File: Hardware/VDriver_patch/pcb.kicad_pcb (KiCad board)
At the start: 4 copper layers, 39.6 x 41.9 mm, 88 parts, among them J501 KAI11002_top, J502 Conn_01x02, J503 Conn_01x02, J504 Conn_01x02, J505 Conn_01x02, J506 Conn_02x05_Odd_Even, U514 1EDN7550B, U515 1EDN7550B, U516 1EDN7550B, U517 1EDN7550B, U518 IRF9389/7309, U519 IRF9389/7309, U520 IRF9389/7309

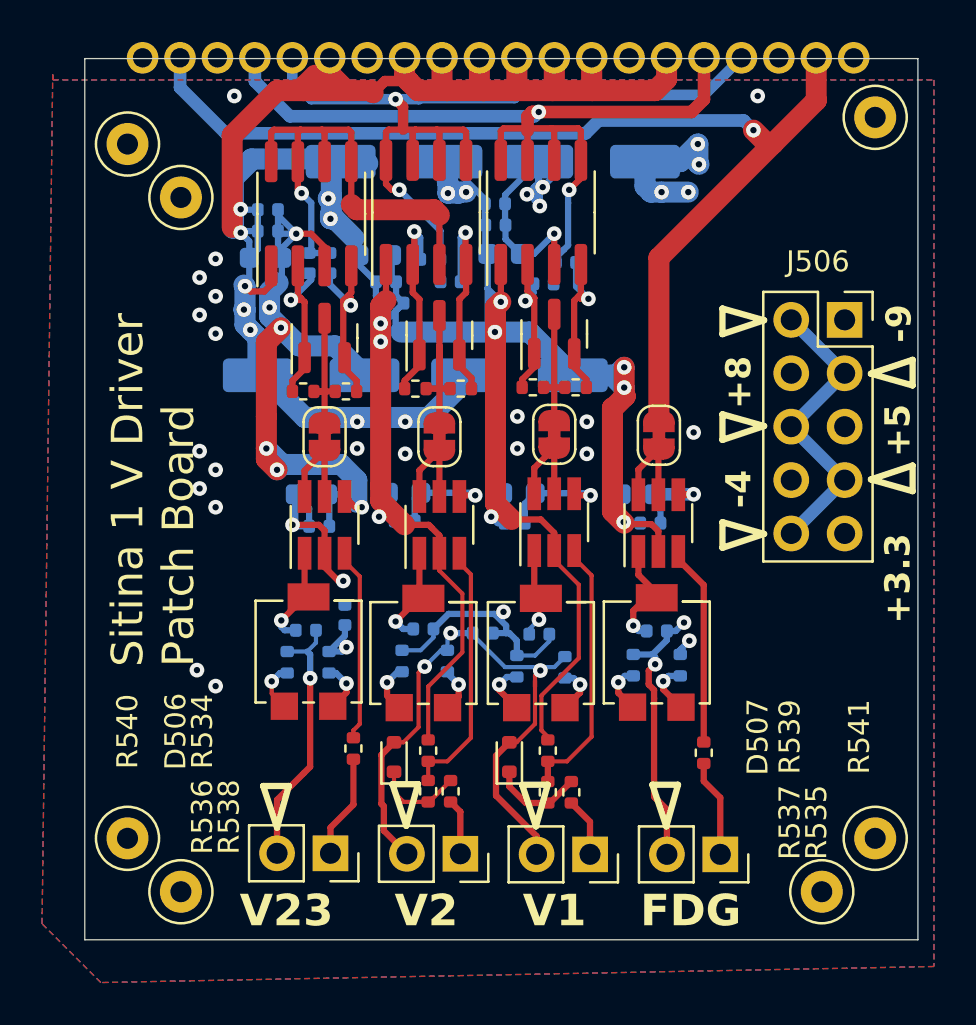
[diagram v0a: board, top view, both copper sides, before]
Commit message: Power Board WIP
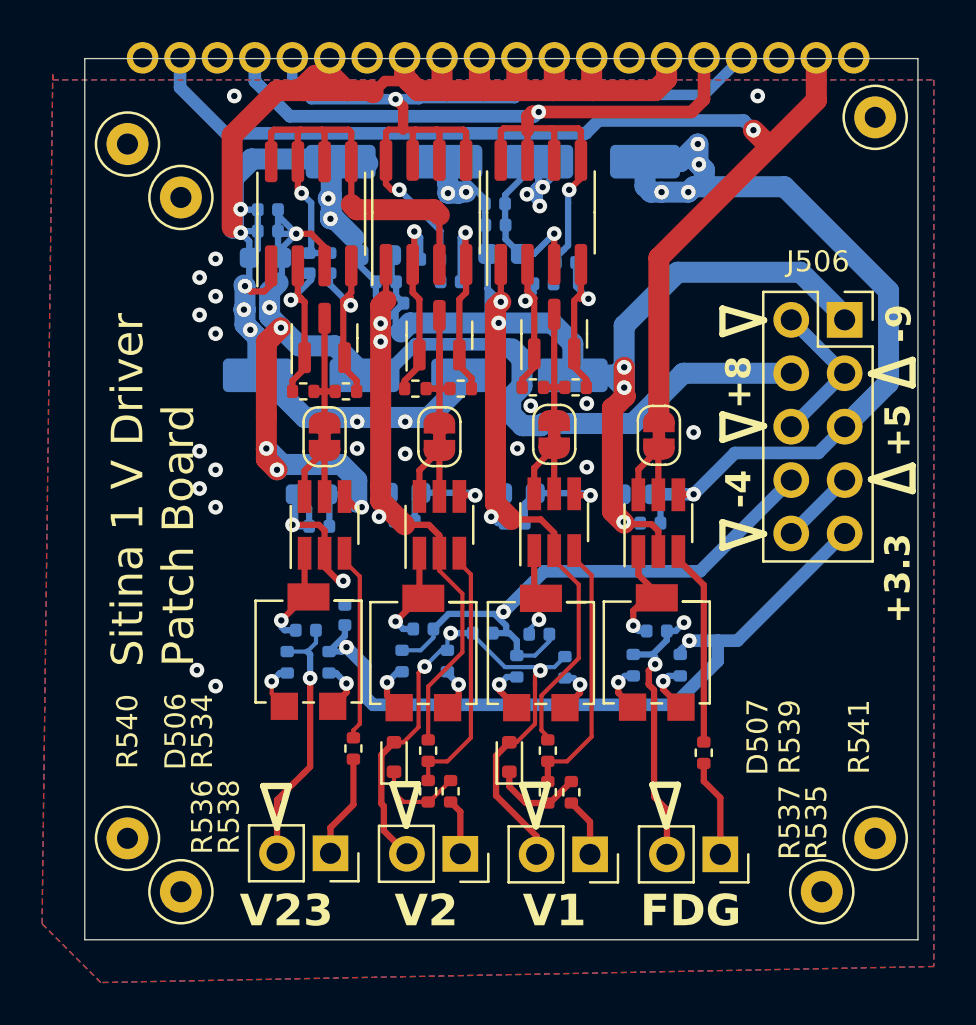
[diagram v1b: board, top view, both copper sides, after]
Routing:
- net +8V: track 35.5 -> 61.3 mm
- net +5V: track 20.7 -> 40.8 mm
- net -9V: track 104.3 -> 120.7 mm
- net +3V3: track 30.0 -> 34.3 mm
- net GND: track 188.1 -> 184.5 mm
- removed copper zone on In1.Cu, net +5V
- removed copper zone on In2.Cu, net +5V
- removed copper zone on In1.Cu, net +8V
- removed copper zone on In2.Cu, net +8V
- removed copper zone on In1.Cu, net -9V
- removed copper zone on In2.Cu, net -9V
- removed copper zone on In1.Cu, net GND
- removed copper zone on In2.Cu, net GND
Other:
- copper layers 4 -> 2
